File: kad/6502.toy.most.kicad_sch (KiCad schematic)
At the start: 8 parts, among them U1 DS1813, U2 6502, U3 28C256, U4 HM62256BLP, U5 HM62256BLP, U6 6551, U7 6522, U8 6522

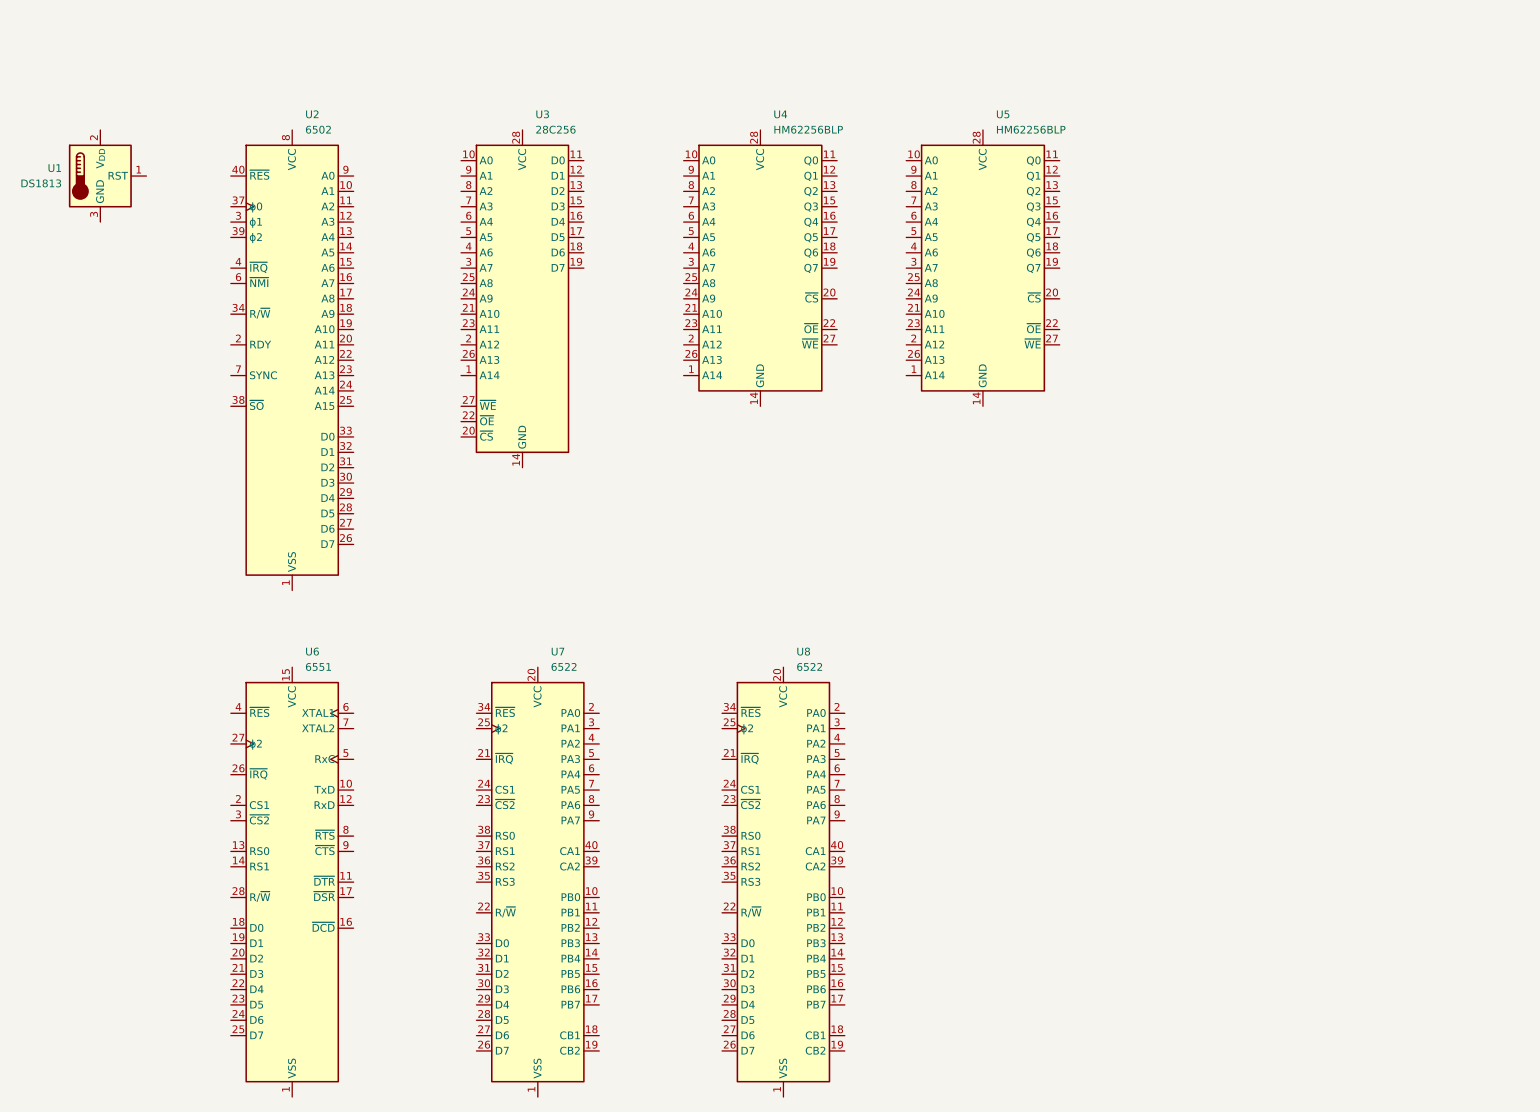
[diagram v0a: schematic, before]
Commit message: update kicad files
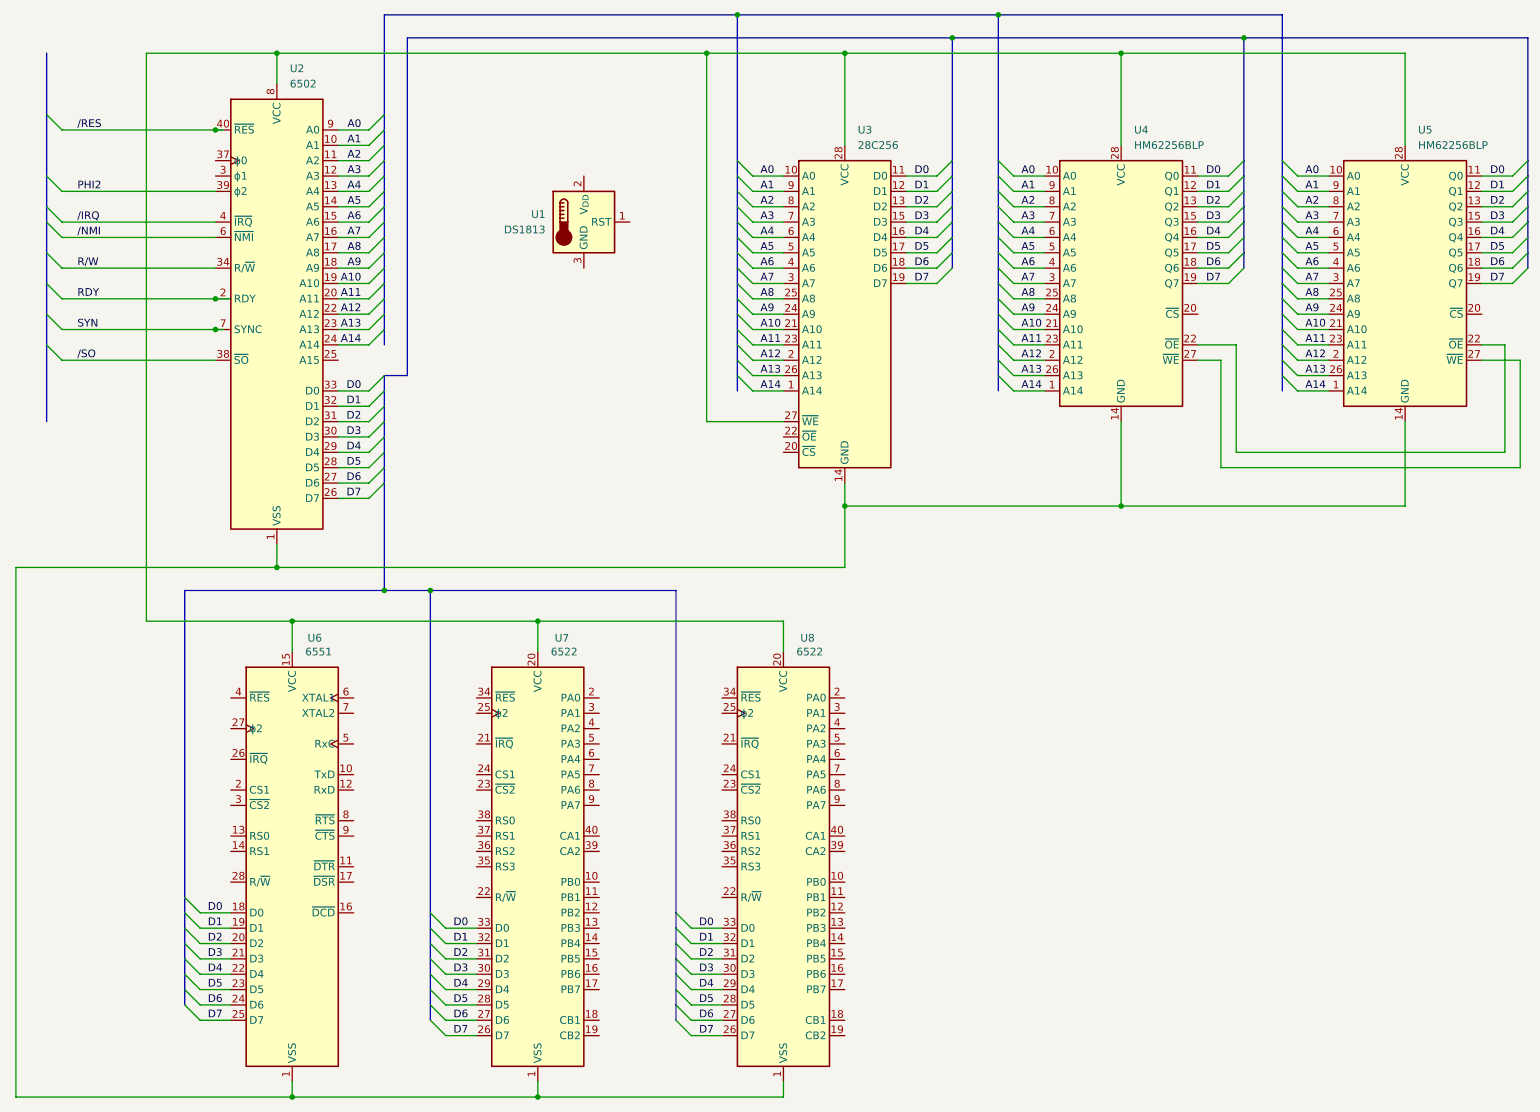
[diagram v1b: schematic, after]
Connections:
- net at U2.1 (VSS), U2.21 (VSS): now also U3.14 (GND), U4.14 (GND), U5.14 (GND), U6.1 (VSS), U7.1 (VSS), U8.1 (VSS)
- net A1: now reaches U2.10 (A1)
- net A1: now also U3.9 (A1), U4.9 (A1), U5.9 (A1)
- net A2: now reaches U2.11 (A2)
- net A2: now also U3.8 (A2), U4.8 (A2), U5.8 (A2)
- net A3: now reaches U2.12 (A3)
- net A3: now also U3.7 (A3), U4.7 (A3), U5.7 (A3)
- net A4: now reaches U2.13 (A4)
- net A4: now also U3.6 (A4), U4.6 (A4), U5.6 (A4)
- net A5: now reaches U2.14 (A5)
- net A5: now also U3.5 (A5), U4.5 (A5), U5.5 (A5)
- net A6: now reaches U2.15 (A6)
- net A6: now also U3.4 (A6), U4.4 (A6), U5.4 (A6)
- net A7: now reaches U2.16 (A7)
- net A7: now also U3.3 (A7), U4.3 (A7), U5.3 (A7)
- net A8: now reaches U2.17 (A8)
- net A8: now also U3.25 (A8), U4.25 (A8), U5.25 (A8)
- net A9: now reaches U2.18 (A9)
- net A9: now also U3.24 (A9), U4.24 (A9), U5.24 (A9)
- net A10: now reaches U2.19 (A10)
- net A10: now also U3.21 (A10), U4.21 (A10), U5.21 (A10)
- net RDY: now reaches U2.2 (RDY)
- net A11: now reaches U2.20 (A11)
- net A11: now also U3.23 (A11), U4.23 (A11), U5.23 (A11)
- net A12: now reaches U2.22 (A12)
- net A12: now also U3.2 (A12), U4.2 (A12), U5.2 (A12)
- net A13: now reaches U2.23 (A13)
- net A13: now also U3.26 (A13), U4.26 (A13), U5.26 (A13)
- net A14: now reaches U2.24 (A14)
- net A14: now also U3.1 (A14), U4.1 (A14), U5.1 (A14)
- net D7: now reaches U2.26 (D7)
- net D7: now also U3.19 (D7), U4.19 (Q7), U5.19 (Q7), U6.25 (D7), U7.26 (D7), U8.26 (D7)
- net D6: now reaches U2.27 (D6)
- net D6: now also U3.18 (D6), U4.18 (Q6), U5.18 (Q6), U6.24 (D6), U7.27 (D6), U8.27 (D6)
- net D5: now reaches U2.28 (D5)
- net D5: now also U3.17 (D5), U4.17 (Q5), U5.17 (Q5), U6.23 (D5), U7.28 (D5), U8.28 (D5)
- net D4: now reaches U2.29 (D4)
- net D4: now also U3.16 (D4), U4.16 (Q4), U5.16 (Q4), U6.22 (D4), U7.29 (D4), U8.29 (D4)
- net D3: now reaches U2.30 (D3)
- net D3: now also U3.15 (D3), U4.15 (Q3), U5.15 (Q3), U6.21 (D3), U7.30 (D3), U8.30 (D3)
- net D2: now reaches U2.31 (D2)
- net D2: now also U3.13 (D2), U4.13 (Q2), U5.13 (Q2), U6.20 (D2), U7.31 (D2), U8.31 (D2)
- net D1: now reaches U2.32 (D1)
- net D1: now also U3.12 (D1), U4.12 (Q1), U5.12 (Q1), U6.19 (D1), U7.32 (D1), U8.32 (D1)
- net D0: now reaches U2.33 (D0)
- net D0: now also U3.11 (D0), U4.11 (Q0), U5.11 (Q0), U6.18 (D0), U7.33 (D0), U8.33 (D0)
- net R/W: now reaches U2.34 (R/~{W})
- net /SO: now reaches U2.38 (~{SO})
- net PHI2: now reaches U2.39 (ϕ2)
- net /IRQ: now reaches U2.4 (~{IRQ})
- net /RES: now reaches U2.40 (~{RES})
- net /NMI: now reaches U2.6 (~{NMI})
- net SYN: now reaches U2.7 (SYNC)
- net at U2.8 (VCC): now also U3.27 (~{WE}), U3.28 (VCC), U4.28 (VCC), U5.28 (VCC), U6.15 (VCC), U7.20 (VCC), U8.20 (VCC)
- net A0: now reaches U2.9 (A0)
- net A0: now also U3.10 (A0), U4.10 (A0), U5.10 (A0)
- net at U5.22 (~{OE}): now also U4.22 (~{OE})
- net at U5.27 (~{WE}): now also U4.27 (~{WE})
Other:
- moved on the sheet: U1, U2, U3, U4, U5, U6, U7, U8
